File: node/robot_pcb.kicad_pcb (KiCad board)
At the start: 2 copper layers, 115.6 x 69.8 mm, 19 parts, among them J1 Conn_01x19_Female, J2 Conn_01x19_Female, J3 esp32Cam, Q1 IRF4905, Q3 IRF4905, Q5 IRF4905, Q7 IRF4905, U1 4N25, U2 4N25, U3 4N25, U4 4N25

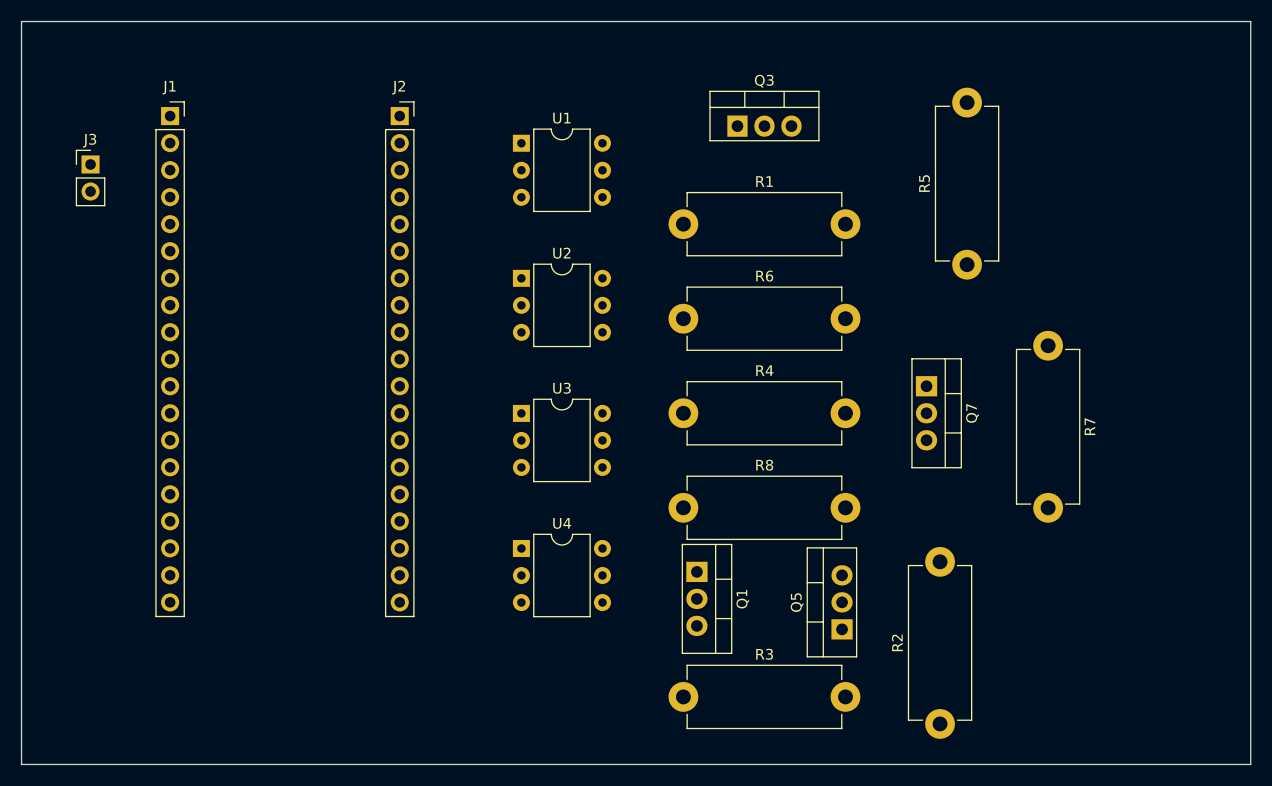
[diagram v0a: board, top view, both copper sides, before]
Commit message: pcb design complete
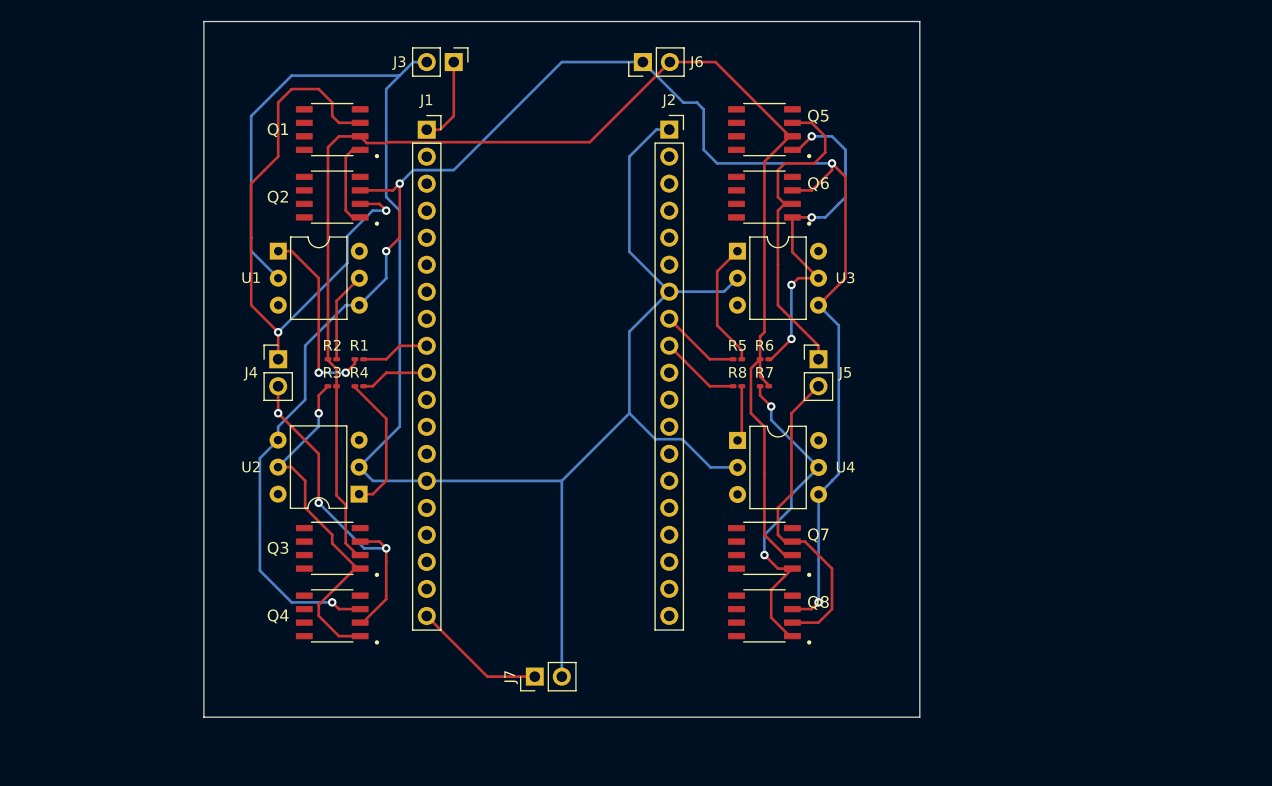
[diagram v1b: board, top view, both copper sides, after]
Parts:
- added J4: motor1, Connector_PinHeader_2.54mm:PinHeader_1x02_P2.54mm_Vertical, F.Cu at (97.8, 88.9)
- added J5: motor2, Connector_PinHeader_2.54mm:PinHeader_1x02_P2.54mm_Vertical, F.Cu at (148.6, 88.9)
- added J6: motor pwr, Connector_PinHeader_2.54mm:PinHeader_1x02_P2.54mm_Vertical, F.Cu at (132.1, 61.0)
- added J7: esp32 pwr, Connector_PinHeader_2.54mm:PinHeader_1x02_P2.54mm_Vertical, F.Cu at (121.9, 118.7)
- added Q2: Q_NMOS_GDS, Downloads:SOIC127P490X600X175-8N, F.Cu at (102.9, 73.7)
- added Q4: Q_NMOS_GDS, Downloads:SOIC127P490X600X175-8N, F.Cu at (102.9, 113.0)
- added Q6: Q_NMOS_GDS, Downloads:SOIC127P490X600X175-8N, F.Cu at (143.5, 73.7)
- added Q8: Q_NMOS_GDS, Downloads:SOIC127P490X600X175-8N, F.Cu at (143.5, 113.0)
- J3: value esp32Cam -> esp32 cam
- Q1, Q3, Q5, Q7: footprint Package_TO_SOT_THT:TO-220-3_Vertical -> Downloads:SOIC127P490X600X175-8N
- R1, R2, R3, R4, R5, R6, R7, R8: footprint Resistor_THT:R_Axial_DIN0614_L14.3mm_D5.7mm_P15.24mm_Horizontal -> Resistor_SMD:R_0201_0603Metric_Pad0.64x0.40mm_HandSolder
- moved R2 66.6 mm to (102.9, 88.9), turned to 180 degrees
- moved Q3 55.0 mm to (102.9, 106.7), turned to 180 degrees
- moved Q1 53.9 mm to (102.9, 67.3), turned to 180 degrees
- moved Q5 47.6 mm to (143.5, 67.3), turned to 180 degrees
- moved R3 44.1 mm to (102.9, 91.4)
- moved J3 35.5 mm to (114.3, 61.0), turned to -90 degrees
- moved R1 33.0 mm to (105.4, 88.9)
- moved R4 30.6 mm to (105.4, 91.4)
- moved R7 26.9 mm to (143.5, 91.4), turned to 0 degrees
- moved U3 25.4 mm to (141.0, 78.7)
- moved U2 25.4 mm to (105.4, 101.6), turned to 180 degrees
- moved J2 25.4 mm to (134.6, 67.3)
- moved U1 25.0 mm to (97.8, 78.7)
- moved J1 24.2 mm to (111.8, 67.3)
- moved R5 23.3 mm to (141.0, 88.9), turned to 180 degrees
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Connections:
- J1 pad 10: unconnected-(J1-Pad10) -> M12
- J1 pad 14: Net-(J3-Pad1) -> ESP_GND
- J1 pad 9: unconnected-(J1-Pad9) -> M11
- J2 pad 1: unconnected-(J2-Pad1) -> ESP_GND
- J2 pad 2: M11 -> unconnected-(J2-Pad2)
- J2 pad 3: M12 -> unconnected-(J2-Pad3)
- J2 pad 4: M21 -> unconnected-(J2-Pad4)
- J2 pad 5: M22 -> unconnected-(J2-Pad5)
- J2 pad 7: unconnected-(J2-Pad7) -> ESP_GND
- J2 pad 8: unconnected-(J2-Pad8) -> M21
- J2 pad 9: unconnected-(J2-Pad9) -> M22
- J3 pad 1: Net-(J3-Pad1) -> /3.3V
- J3 pad 2: /3.3V -> ESP_GND
- Q1 pad 3: Net-(M5-Pad1) -> MO1
- Q3 pad 3: Net-(M1-Pad1) -> MO2
- Q5 pad 1: Net-(R3-Pad1) -> Net-(Q5-Pad1)
- Q5 pad 3: Net-(M5-Pad2) -> MO3
- Q7 pad 3: Net-(M1-Pad2) -> MO4
- R1 pad 2: /3.3V -> M11
- R3 pad 1: Net-(R3-Pad1) -> Net-(Q3-Pad1)
- R4 pad 2: /3.3V -> M12
- R5 pad 2: /3.3V -> M21
- R6 pad 1: Net-(Q3-Pad1) -> Net-(Q5-Pad1)
- R8 pad 2: /3.3V -> M22
- U1 pad 2: M11 -> ESP_GND
- U1 pad 4: Net-(Q2-Pad3) -> MGND
- U2 pad 1: Net-(R5-Pad1) -> Net-(R4-Pad1)
- U2 pad 2: M21 -> ESP_GND
- U2 pad 4: Net-(Q4-Pad3) -> MGND
- U3 pad 1: Net-(R4-Pad1) -> Net-(R5-Pad1)
- U3 pad 2: M12 -> ESP_GND
- U3 pad 4: Net-(Q2-Pad3) -> MGND
- U3 pad 5: Net-(R3-Pad1) -> Net-(Q5-Pad1)
- U4 pad 2: M22 -> ESP_GND
- U4 pad 4: Net-(Q4-Pad3) -> MGND
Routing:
- net ESP_GND: track 0.00 -> 172.6 mm
- net MGND: track 0.00 -> 161.6 mm, vias 0 -> 5
- net /Vm: track 0.00 -> 136.2 mm
- net MO1: track 0.00 -> 55.6 mm, vias 0 -> 2
- net Net-(Q3-Pad1): track 0.00 -> 34.2 mm, vias 0 -> 1
- net Net-(Q5-Pad1): track 0.00 -> 33.8 mm, vias 0 -> 4
- net MO2: track 0.00 -> 31.8 mm, vias 0 -> 3
- net Net-(Q7-Pad1): track 0.00 -> 31.6 mm, vias 0 -> 2
- net MO3: track 0.00 -> 30.9 mm
- net MO4: track 0.00 -> 30.0 mm
- net Net-(R1-Pad1): track 0.00 -> 17.9 mm, vias 0 -> 2
- net Net-(Q1-Pad1): track 0.00 -> 16.8 mm
- net Net-(R4-Pad1): track 0.00 -> 13.2 mm
- net /Vcc: track 0.00 -> 12.5 mm
- net Net-(R5-Pad1): track 0.00 -> 11.9 mm
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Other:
- board size 115.6 x 69.8 mm -> 67.3 x 65.4 mm
